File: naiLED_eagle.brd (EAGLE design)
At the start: 12.4 x 14 mm, 8 parts, among them U1 AT24C256C-MAHL-T, U3 ATTINY85-20SU

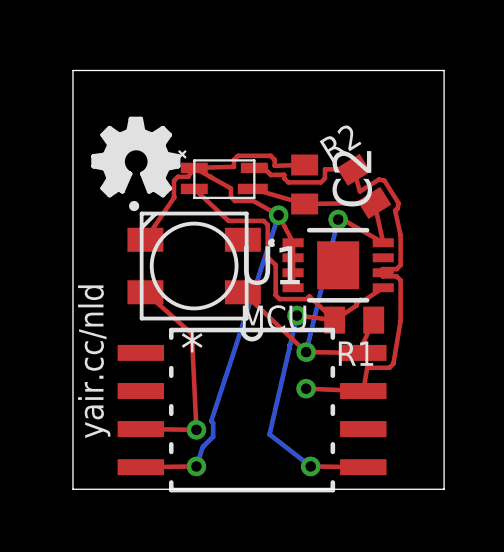
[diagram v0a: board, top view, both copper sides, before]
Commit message: layout, meh
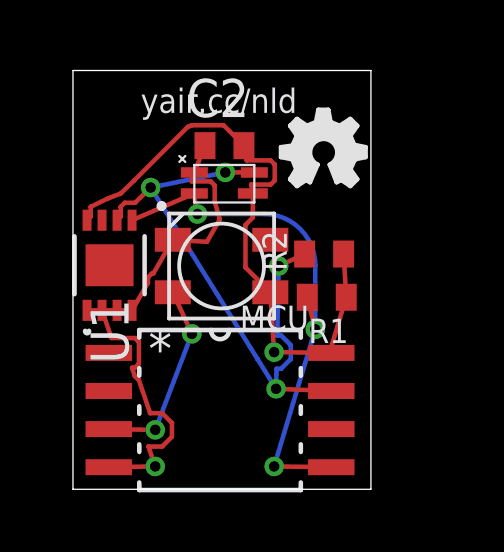
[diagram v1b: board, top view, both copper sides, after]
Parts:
- moved U1 7.62 mm to (1.22, 7.47), turned to 90 degrees
- moved E$1 6.26 mm to (6.93, 10.1)
- moved C2 2.97 mm to (5.05, 11.5), turned to 0 degrees
- moved R2 2.62 mm to (8.37, 7.84), turned to 0 degrees
- moved R1 1.19 mm to (8.46, 6.40)
- moved U3 1.07 mm to (4.90, 2.64)
- moved U$1 0.91 mm to (4.95, 7.44)
- moved U$2 0.15 mm to (5.08, 10.2)
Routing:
- net GND: track 24.2 -> 18.7 mm, vias 2 -> 1
- net D2/A1/SCK/SCL: track 16.7 -> 21.1 mm, vias 1 -> 4
- net VCC: track 17.7 -> 21.1 mm, vias 2 -> 1
- net D0/PWM/MOSI/SDA: track 18.6 -> 17.6 mm, vias 2 -> 3
- net D4/PWM: track 7.44 -> 6.50 mm, vias 1 -> 2
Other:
- board size 12.4 x 14 mm -> 9.9 x 14 mm

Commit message: auditing
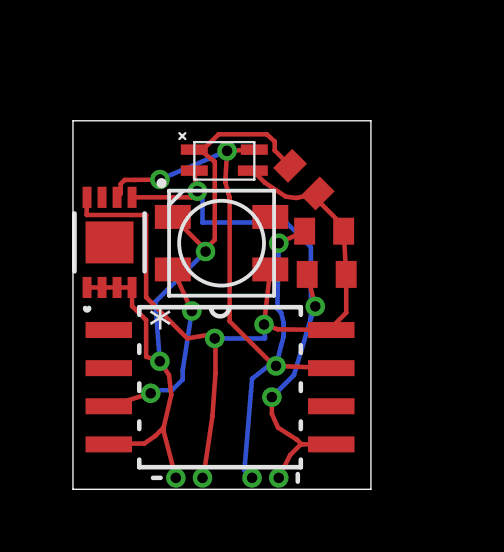
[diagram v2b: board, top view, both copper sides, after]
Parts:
- moved E$1 2.96 mm to (6.32, 7.21), flipped to the bottom
- moved C2 2.88 mm to (7.70, 10.3), turned to 315 degrees
- moved R2 0.76 mm to (8.37, 8.60)
- moved U$1 0.76 mm to (4.95, 8.20)
- moved U3 0.76 mm to (4.90, 3.40)
- moved R1 0.76 mm to (8.46, 7.16)
- moved U1 0.76 mm to (1.22, 8.23)
- moved U$2 0.76 mm to (5.08, 11.0)
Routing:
- net VCC: track 21.1 -> 27.1 mm, vias 1 -> 3
- net GND: track 18.7 -> 24.3 mm, vias 1 -> 3
- net D2/A1/SCK/SCL: track 21.1 -> 24.8 mm, vias 4 -> 5
- net D0/PWM/MOSI/SDA: track 17.6 -> 19.4 mm, vias 3 -> 4
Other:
- board size 9.9 x 14 mm -> 9.9 x 12.3 mm
- board text removed: "MCU"
